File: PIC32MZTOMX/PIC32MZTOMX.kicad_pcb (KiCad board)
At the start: 2 copper layers, 85.7 x 94.5 mm, 88 parts, among them J101 Conn_02x08_Odd_Even, J102 Conn_02x08_Odd_Even, J103 Conn_02x08_Odd_Even, J104 Conn_02x08_Odd_Even, U101 PIC32MZ2048ECM064, U102 REF3033, Y101 8Mhz, Y102 12Mhz

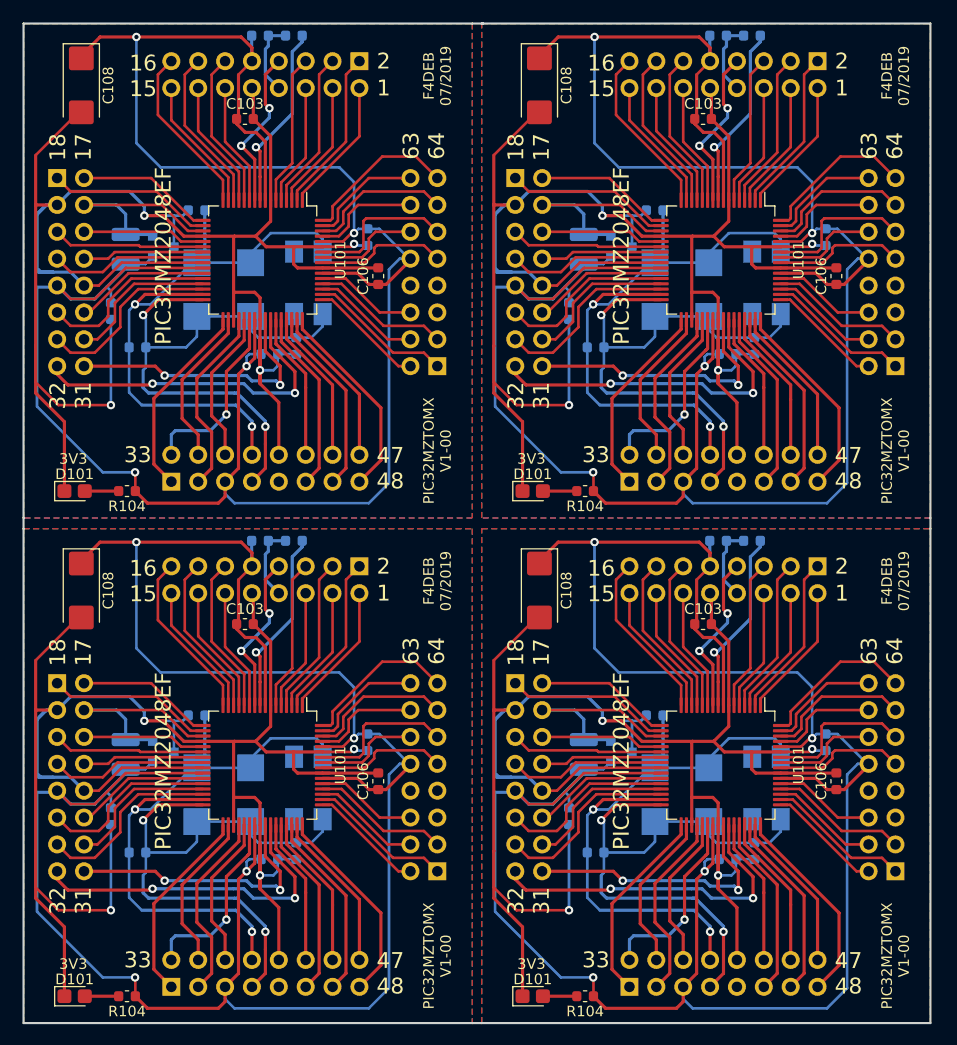
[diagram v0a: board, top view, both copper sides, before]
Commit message: MAJ HALF DUPLEX
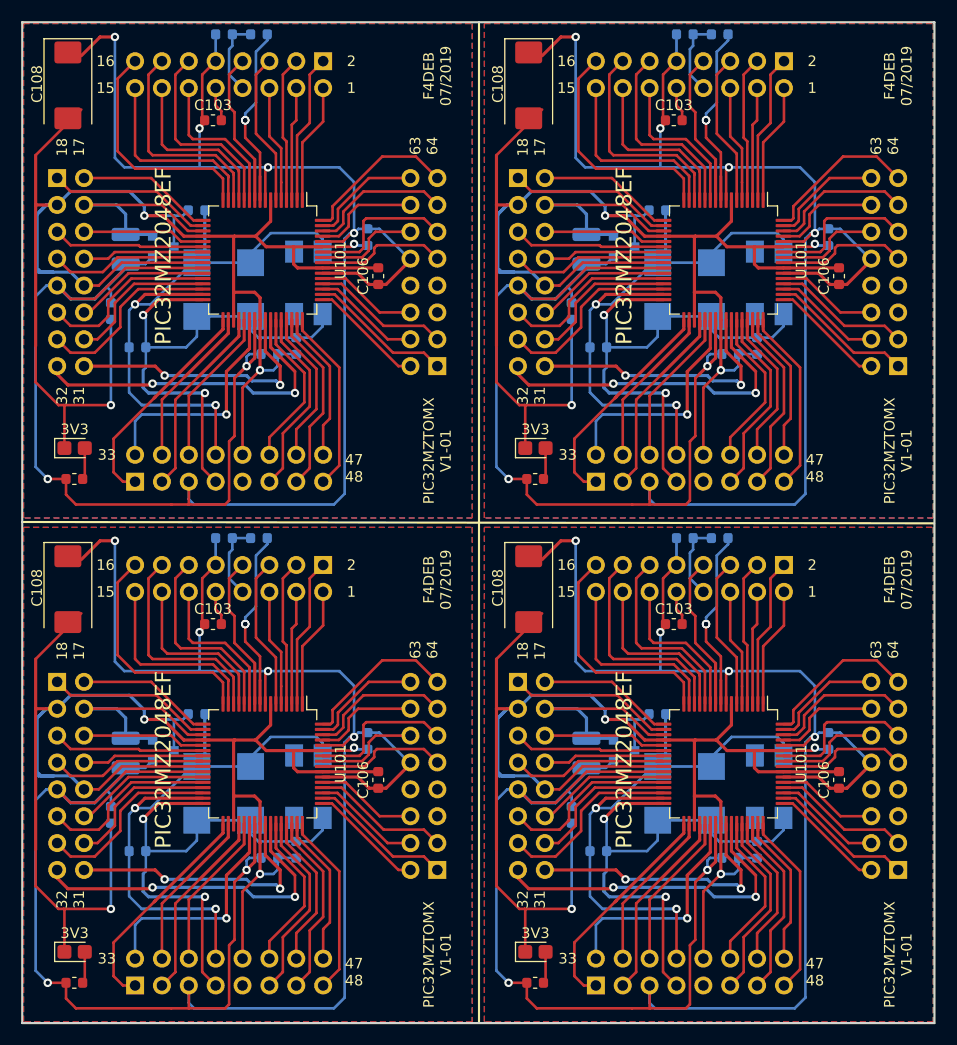
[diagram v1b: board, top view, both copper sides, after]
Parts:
- removed the C101 at (186.5, 127.0)
- removed the C101 at (143.2, 127.0)
- removed the C101 at (186.5, 79.2)
- removed the C102 at (152.7, 139.8)
- removed the C102 at (196.0, 139.8)
- removed the C102 at (196.0, 92.1)
- removed the C103 at (191.1, 118.4)
- removed the C103 at (147.8, 118.4)
- removed the C103 at (191.1, 70.6)
- removed the C104 at (178.4, 136.5)
- removed the C104 at (135.1, 136.5)
- removed the C104 at (178.4, 88.8)
- removed the C105 at (159.4, 129.5)
- removed the C105 at (202.7, 129.5)
- removed the C105 at (202.7, 81.8)
- removed the C106 at (203.7, 133.2)
- removed the C106 at (160.4, 133.2)
- removed the C106 at (203.7, 85.5)
- removed the C107 at (193.4, 140.6)
- removed the C107 at (150.1, 140.6)
- removed the C107 at (193.4, 92.8)
- removed the C108 at (175.6, 115.2)
- removed the C108 at (132.3, 115.2)
- removed the C108 at (175.6, 67.4)
- removed the D101 at (131.7, 153.5)
- removed the D101 at (175.0, 153.5)
- removed the D101 at (175.0, 105.8)
- removed the J101 at (158.6, 112.9)
- removed the J101 at (201.9, 112.9)
- removed the J101 at (201.9, 65.2)
- removed the J102 at (173.4, 124.0)
- removed the J102 at (130.0, 124.0)
- removed the J102 at (173.4, 76.2)
- removed the J103 at (140.8, 152.7)
- removed the J103 at (184.2, 152.7)
- removed the J103 at (184.2, 104.9)
- removed the J104 at (209.3, 141.7)
- removed the J104 at (166.0, 141.7)
- removed the J104 at (209.3, 94.0)
- removed the L101 at (179.8, 130.7)
- removed the L101 at (136.5, 130.7)
- removed the L101 at (179.8, 82.9)
- removed the R101 at (180.9, 140.0)
- removed the R101 at (137.6, 140.0)
- removed the R101 at (180.9, 92.2)
- removed the R102 at (195.7, 110.5)
- removed the R102 at (152.4, 110.5)
- removed the R102 at (195.7, 62.7)
- removed the R103 at (149.2, 110.5)
- removed the R103 at (192.5, 110.5)
- removed the R103 at (192.5, 62.7)
- removed the R104 at (136.7, 153.5)
- removed the R104 at (180.0, 153.5)
- removed the R104 at (180.0, 105.8)
- removed the U101 at (149.5, 131.7)
- removed the U101 at (192.8, 131.7)
- removed the U101 at (192.8, 83.9)
- removed the U102 at (183.4, 130.4)
- removed the U102 at (140.1, 130.4)
- removed the U102 at (183.4, 82.7)
- removed the Y101 at (189.1, 134.5)
- removed the Y101 at (145.8, 134.5)
- removed the Y101 at (189.1, 86.7)
- removed the Y102 at (153.8, 133.9)
- removed the Y102 at (197.1, 133.9)
- removed the Y102 at (197.1, 86.1)
- added C101: 22pf, Capacitor_SMD:C_0603_1608Metric, B.Cu at (143.2, 126.9)
- added C101: 22pf, Capacitor_SMD:C_0603_1608Metric, B.Cu at (186.8, 126.9)
- added C101: 22pf, Capacitor_SMD:C_0603_1608Metric, B.Cu at (186.8, 79.2)
- added C102: 22pf, Capacitor_SMD:C_0603_1608Metric, B.Cu at (152.7, 139.7)
- added C102: 22pf, Capacitor_SMD:C_0603_1608Metric, B.Cu at (196.2, 139.7)
- added C102: 22pf, Capacitor_SMD:C_0603_1608Metric, B.Cu at (196.2, 92.1)
- added C103: C, Capacitor_SMD:C_0603_1608Metric, F.Cu at (144.8, 118.4)
- added C103: C, Capacitor_SMD:C_0603_1608Metric, F.Cu at (188.3, 118.4)
- added C103: C, Capacitor_SMD:C_0603_1608Metric, F.Cu at (188.3, 70.7)
- added C104: C, Capacitor_SMD:C_0603_1608Metric, B.Cu at (135.1, 136.4)
- added C104: C, Capacitor_SMD:C_0603_1608Metric, B.Cu at (178.7, 136.4)
- added C104: C, Capacitor_SMD:C_0603_1608Metric, B.Cu at (178.7, 88.8)
- added C105: C, Capacitor_SMD:C_0603_1608Metric, B.Cu at (159.4, 129.4)
- added C105: C, Capacitor_SMD:C_0603_1608Metric, B.Cu at (202.9, 129.4)
- added C105: C, Capacitor_SMD:C_0603_1608Metric, B.Cu at (202.9, 81.8)
- added C106: C, Capacitor_SMD:C_0603_1608Metric, F.Cu at (160.4, 133.1)
- added C106: C, Capacitor_SMD:C_0603_1608Metric, F.Cu at (204.0, 133.1)
- added C106: C, Capacitor_SMD:C_0603_1608Metric, F.Cu at (204.0, 85.5)
- added C107: C, Capacitor_SMD:C_0603_1608Metric, B.Cu at (150.1, 140.5)
- added C107: C, Capacitor_SMD:C_0603_1608Metric, B.Cu at (193.7, 140.5)
- added C107: C, Capacitor_SMD:C_0603_1608Metric, B.Cu at (193.7, 92.8)
- added C108: CP, Capacitor_Tantalum_SMD:CP_EIA-7343-20_Kemet-V, F.Cu at (174.6, 115.1)
- added C108: CP, Capacitor_Tantalum_SMD:CP_EIA-7343-20_Kemet-V, F.Cu at (131.1, 115.1)
- added C108: CP, Capacitor_Tantalum_SMD:CP_EIA-7343-20_Kemet-V, F.Cu at (174.6, 67.4)
- added D101: LED, LED_SMD:LED_0805_2012Metric_Castellated, F.Cu at (131.7, 149.4)
- added D101: LED, LED_SMD:LED_0805_2012Metric_Castellated, F.Cu at (175.3, 149.4)
- added D101: LED, LED_SMD:LED_0805_2012Metric_Castellated, F.Cu at (175.3, 101.7)
- added J101: Conn_02x08_Odd_Even, Connector_PinSocket_2.54mm:PinSocket_2x08_P2.54mm_Vertical, B.Cu at (155.2, 112.8)
- added J101: Conn_02x08_Odd_Even, Connector_PinSocket_2.54mm:PinSocket_2x08_P2.54mm_Vertical, B.Cu at (198.8, 112.8)
- added J101: Conn_02x08_Odd_Even, Connector_PinSocket_2.54mm:PinSocket_2x08_P2.54mm_Vertical, B.Cu at (198.8, 65.2)
- added J102: Conn_02x08_Odd_Even, Connector_PinSocket_2.54mm:PinSocket_2x08_P2.54mm_Vertical, B.Cu at (130.0, 123.8)
- added J102: Conn_02x08_Odd_Even, Connector_PinSocket_2.54mm:PinSocket_2x08_P2.54mm_Vertical, B.Cu at (173.6, 123.8)
- added J102: Conn_02x08_Odd_Even, Connector_PinSocket_2.54mm:PinSocket_2x08_P2.54mm_Vertical, B.Cu at (173.6, 76.2)
- added J103: Conn_02x08_Odd_Even, Connector_PinSocket_2.54mm:PinSocket_2x08_P2.54mm_Vertical, B.Cu at (137.4, 152.5)
- added J103: Conn_02x08_Odd_Even, Connector_PinSocket_2.54mm:PinSocket_2x08_P2.54mm_Vertical, B.Cu at (181.0, 152.5)
- added J103: Conn_02x08_Odd_Even, Connector_PinSocket_2.54mm:PinSocket_2x08_P2.54mm_Vertical, B.Cu at (181.0, 104.9)
- added J104: Conn_02x08_Odd_Even, Connector_PinSocket_2.54mm:PinSocket_2x08_P2.54mm_Vertical, B.Cu at (209.6, 141.6)
- added J104: Conn_02x08_Odd_Even, Connector_PinSocket_2.54mm:PinSocket_2x08_P2.54mm_Vertical, B.Cu at (166.0, 141.6)
- added J104: Conn_02x08_Odd_Even, Connector_PinSocket_2.54mm:PinSocket_2x08_P2.54mm_Vertical, B.Cu at (209.6, 94.0)
- added L101: INDUCTOR, Inductor_SMD:L_1210_3225Metric, B.Cu at (180.1, 130.6)
- added L101: INDUCTOR, Inductor_SMD:L_1210_3225Metric, B.Cu at (136.5, 130.6)
- added L101: INDUCTOR, Inductor_SMD:L_1210_3225Metric, B.Cu at (180.1, 82.9)
- added R101: 1M, Resistor_SMD:R_0603_1608Metric, B.Cu at (181.2, 139.8)
- added R101: 1M, Resistor_SMD:R_0603_1608Metric, B.Cu at (137.6, 139.8)
- added R101: 1M, Resistor_SMD:R_0603_1608Metric, B.Cu at (181.2, 92.2)
- added R102: 470, Resistor_SMD:R_0603_1608Metric, B.Cu at (192.7, 110.2)
- added R102: 470, Resistor_SMD:R_0603_1608Metric, B.Cu at (149.1, 110.2)
- added R102: 470, Resistor_SMD:R_0603_1608Metric, B.Cu at (192.7, 62.6)
- added R103: 10k, Resistor_SMD:R_0603_1608Metric, B.Cu at (189.4, 110.2)
- added R103: 10k, Resistor_SMD:R_0603_1608Metric, B.Cu at (145.8, 110.2)
- added R103: 10k, Resistor_SMD:R_0603_1608Metric, B.Cu at (189.4, 62.6)
- added R104: 1k, Resistor_SMD:R_0603_1608Metric, F.Cu at (131.7, 152.3)
- added R104: 1k, Resistor_SMD:R_0603_1608Metric, F.Cu at (175.2, 152.3)
- added R104: 1k, Resistor_SMD:R_0603_1608Metric, F.Cu at (175.2, 104.6)
- added U101: PIC32MZ2048ECM064, Package_QFP:TQFP-64_10x10mm_P0.5mm, F.Cu at (149.5, 131.6)
- added U101: PIC32MZ2048ECM064, Package_QFP:TQFP-64_10x10mm_P0.5mm, F.Cu at (193.0, 131.6)
- added U101: PIC32MZ2048ECM064, Package_QFP:TQFP-64_10x10mm_P0.5mm, F.Cu at (193.0, 83.9)
- added U102: REF3033, Package_TO_SOT_SMD:SOT-23, B.Cu at (140.1, 130.3)
- added U102: REF3033, Package_TO_SOT_SMD:SOT-23, B.Cu at (183.6, 130.3)
- added U102: REF3033, Package_TO_SOT_SMD:SOT-23, B.Cu at (183.6, 82.7)
- added Y101: 8Mhz, f4deb-mod-library:QTZ, B.Cu at (145.8, 134.4)
- added Y101: 8Mhz, f4deb-mod-library:QTZ, B.Cu at (189.4, 134.4)
- added Y101: 8Mhz, f4deb-mod-library:QTZ, B.Cu at (189.4, 86.7)
- added Y102: 12Mhz, Crystal:Crystal_SMD_7050-4Pin_7.0x5.0mm, B.Cu at (197.4, 133.7)
- added Y102: 12Mhz, Crystal:Crystal_SMD_7050-4Pin_7.0x5.0mm, B.Cu at (153.8, 133.7)
- added Y102: 12Mhz, Crystal:Crystal_SMD_7050-4Pin_7.0x5.0mm, B.Cu at (197.4, 86.1)
- C108: footprint Capacitor_Tantalum_SMD:CP_EIA-6032-15_Kemet-U_Pad2.25x2.35mm_HandSolder -> Capacitor_Tantalum_SMD:CP_EIA-7343-20_Kemet-V
- moved R104 5.11 mm to (131.7, 104.6), turned to 0 degrees
- moved D101 4.06 mm to (131.7, 101.7)
- moved J101 3.43 mm to (155.2, 65.2)
- moved J103 3.43 mm to (137.4, 104.9)
- moved R103 3.41 mm to (145.8, 62.6)
- moved R102 3.30 mm to (149.1, 62.6)
- moved C103 3.03 mm to (144.8, 70.7)
- moved C108 1.27 mm to (131.1, 67.4)
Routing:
- net /20: track 757.1 -> 662.2 mm
- net /10: track 878.9 -> 851.7 mm, vias 16 -> 24
- net /16: track 64.8 -> 89.0 mm
- net /15: track 51.3 -> 73.0 mm
- net /14: track 62.3 -> 82.0 mm
- net /13: track 48.7 -> 65.7 mm
- net /33: track 71.0 -> 87.7 mm
- net /40: track 218.6 -> 202.4 mm
- net /12: track 59.7 -> 74.3 mm
- net /11: track 46.2 -> 59.0 mm
- net /34: track 74.7 -> 85.1 mm
- net /39: track 257.6 -> 247.4 mm
- net /48: track 76.8 -> 69.5 mm
- net /1: track 51.3 -> 45.6 mm
- net /2: track 62.3 -> 56.6 mm
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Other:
- board size 85.7 x 94.5 mm -> 86.2 x 94.6 mm
- board text added: "15"
- board text added: "16"
- board text added: "PIC32MZTOMX V1-01"
- board text removed: "16 15"
- board text removed: "PIC32MZTOMX V1-00"
